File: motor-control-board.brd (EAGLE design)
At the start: 23.9 x 27.7 mm, 28 parts, among them U1 DRV8830, U2 DRV8830, U3 DRV8830, U4 DRV8830

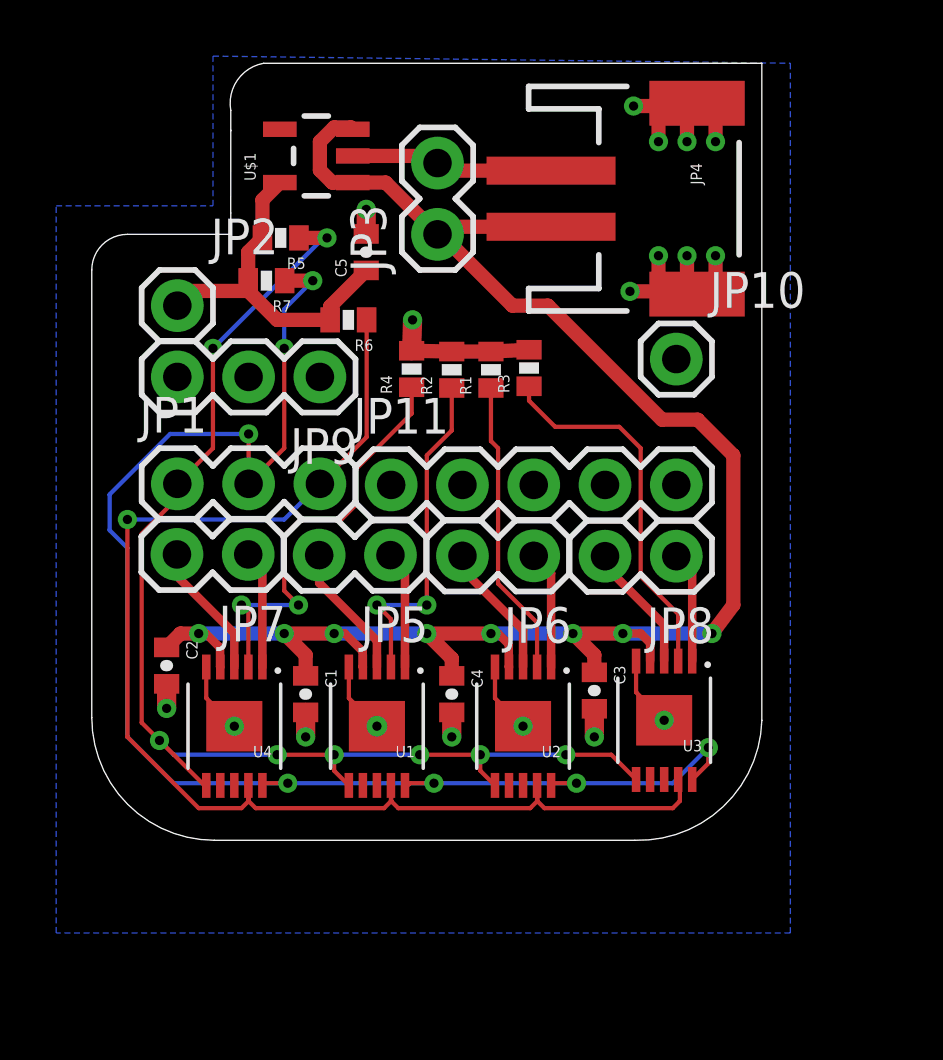
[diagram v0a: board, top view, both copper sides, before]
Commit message: Before adding 0805 resistors
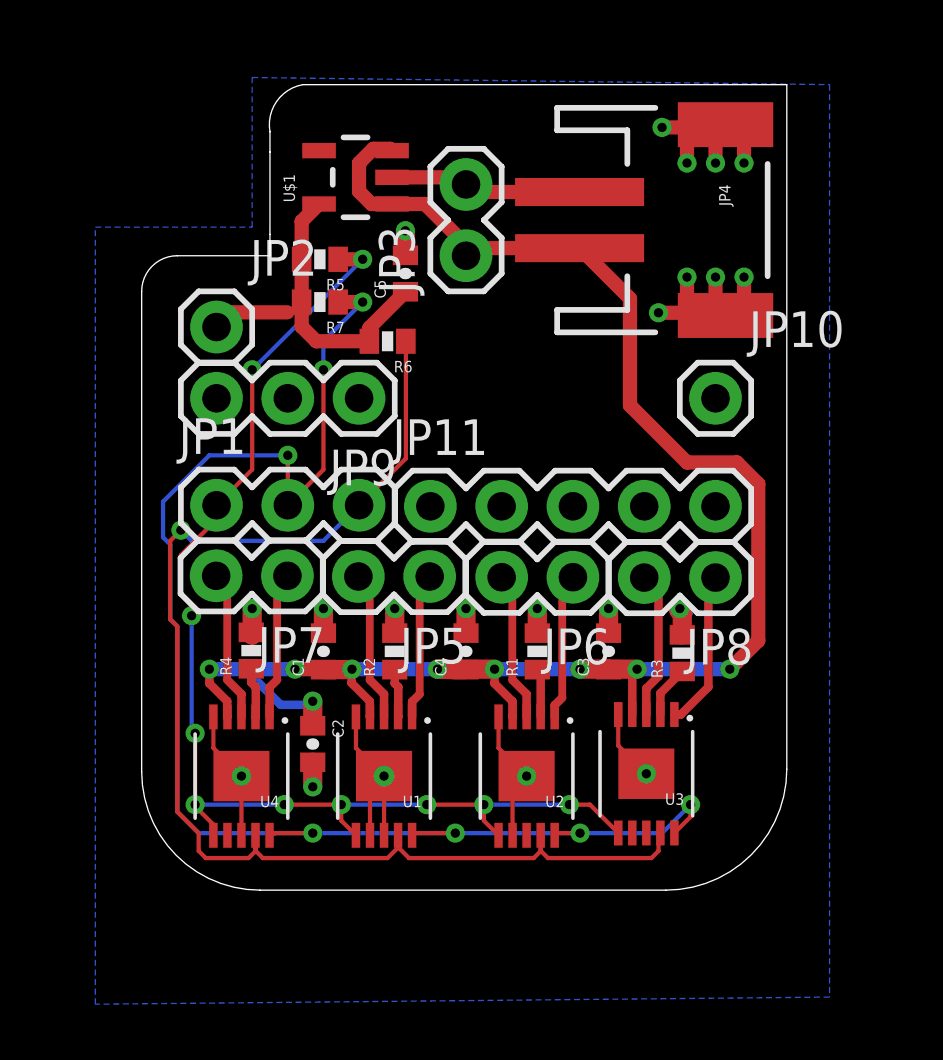
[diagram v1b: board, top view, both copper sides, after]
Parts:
- moved R4 11.5 mm to (3.90, 8.54)
- moved R3 11.5 mm to (19.3, 8.44)
- moved R2 10.2 mm to (9.02, 8.51)
- moved R1 10.2 mm to (14.1, 8.51)
- moved C2 5.91 mm to (6.10, 5.21)
- moved R7 2.05 mm to (6.35, 21.0)
- moved U3 2.01 mm to (18.0, 4.15)
- moved JP10 1.98 mm to (20.4, 17.5)
- moved U1 1.80 mm to (8.64, 4.06)
- moved U4 1.80 mm to (3.56, 4.06)
- moved U2 1.78 mm to (13.7, 4.06)
- moved C1 1.65 mm to (6.48, 8.51), turned to 90 degrees
- moved C4 1.61 mm to (11.6, 8.51), turned to 90 degrees
- moved C5 1.59 mm to (9.40, 22.0)
- moved JP11 1.59 mm to (10.3, 13.7)
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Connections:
- removed net N$1: U1.7, U1.8, U2.7, U4.8
- net GND: now also U1.7, U1.8, U2.7, U4.8
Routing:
- net N$5: track 15.0 -> 1.78 mm, vias 2 -> 0
- net N$3: track 13.3 -> 1.86 mm
- net N$2: track 12.3 -> 1.74 mm, vias 2 -> 0
- net N$4: track 10.6 -> 1.71 mm
- net GND: track 27.2 -> 34.4 mm, vias 10 -> 13
- net MOTOR4_B: track 3.97 -> 5.62 mm
- net !FAULT: track 44.5 -> 42.9 mm, vias 8 -> 10
- net MOTOR2_B: track 4.22 -> 5.29 mm
- net MOTOR1_B: track 4.20 -> 5.26 mm
- net MOTOR3_B: track 4.22 -> 5.25 mm
- net VCC: track 64.0 -> 63.1 mm, vias 8 -> 9
- net MOTOR4_A: track 4.61 -> 5.27 mm
- net MOTOR2_A: track 4.86 -> 5.40 mm
- net MOTOR1_A: track 4.84 -> 5.38 mm
- net SDA: track 47.3 -> 46.8 mm
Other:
- board size 23.9 x 27.7 mm -> 23 x 28.7 mm

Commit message: -
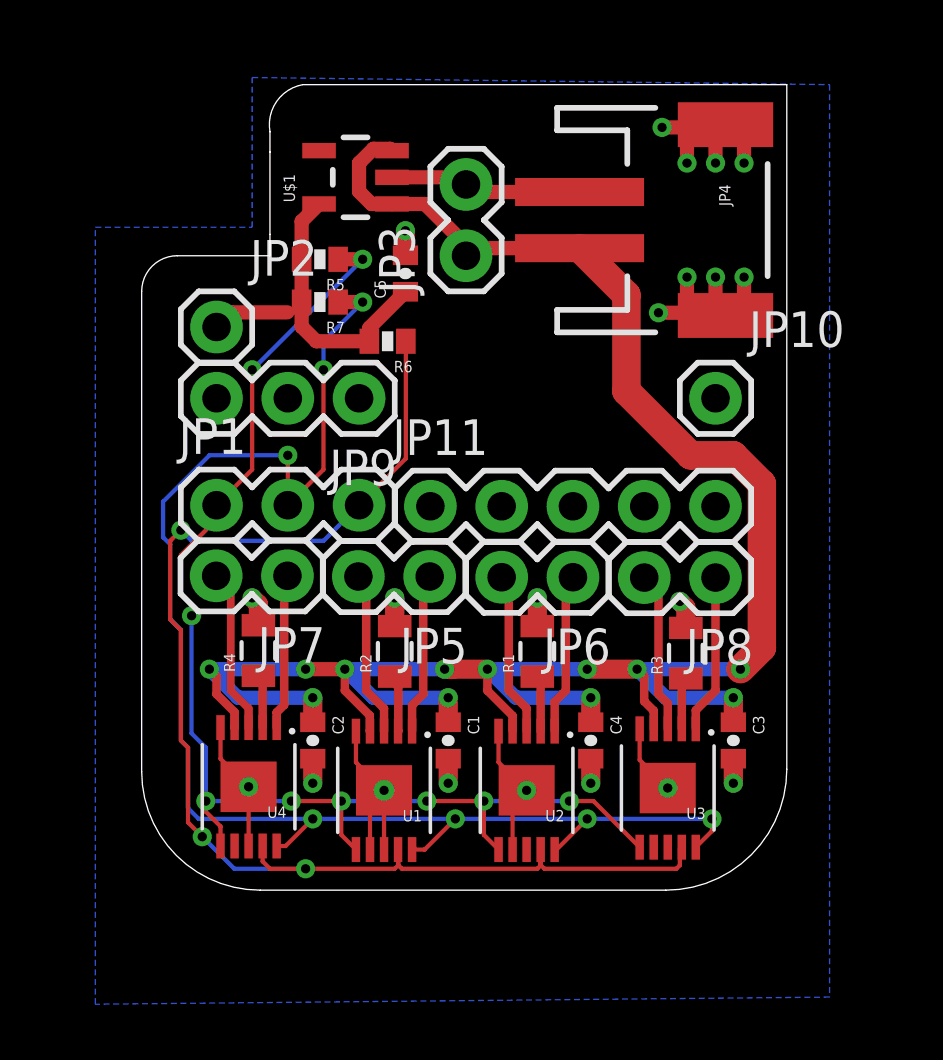
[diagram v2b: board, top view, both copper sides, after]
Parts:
- R1, R2, R3, R4: device SparkFun-Resistors:0402-RES -> SparkFun-Resistors:0805
- moved C1 5.46 mm to (10.9, 5.33), turned to 270 degrees
- moved C3 5.46 mm to (21.1, 5.33), turned to 270 degrees
- moved C4 5.46 mm to (16.0, 5.33), turned to 270 degrees
- moved U3 0.92 mm to (18.7, 3.64)
- moved U1 0.51 mm to (8.64, 3.56)
- moved U2 0.51 mm to (13.7, 3.56)
- moved U4 0.46 mm to (3.81, 3.68)
- moved R4 0.25 mm to (4.16, 8.54)
- moved R3 0.13 mm to (19.4, 8.44)
- moved C2 0.13 mm to (6.10, 5.33)
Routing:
- net VCC: track 63.1 -> 79.6 mm, vias 9 -> 12
- net !FAULT: track 42.9 -> 45.1 mm, vias 10 -> 9
- net SDA: track 46.8 -> 48.5 mm, vias 1 -> 3
- net SCL: track 51.7 -> 52.9 mm
- net GND: track 34.4 -> 35.3 mm
- net MOTOR3_B: track 5.25 -> 5.75 mm
- net MOTOR3_A: track 5.35 -> 5.85 mm
- net MOTOR1_B: track 5.26 -> 5.77 mm
- net MOTOR1_A: track 5.38 -> 5.89 mm
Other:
- board text added: "+"
- board text added: "-"
- board text added: "LightBlue Bean H-bridge motor controller"
- board text added: "MOTOR 1"
- board text added: "MOTOR 2"
- board text added: "MOTOR 3"
- board text added: "MOTOR 4"
- board text removed: "GND"
